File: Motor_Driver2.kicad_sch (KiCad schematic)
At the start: 20 parts, among them J701 Conn_01x02_Socket, U701 DMHT6016LFJ-13, U702 DRV8701

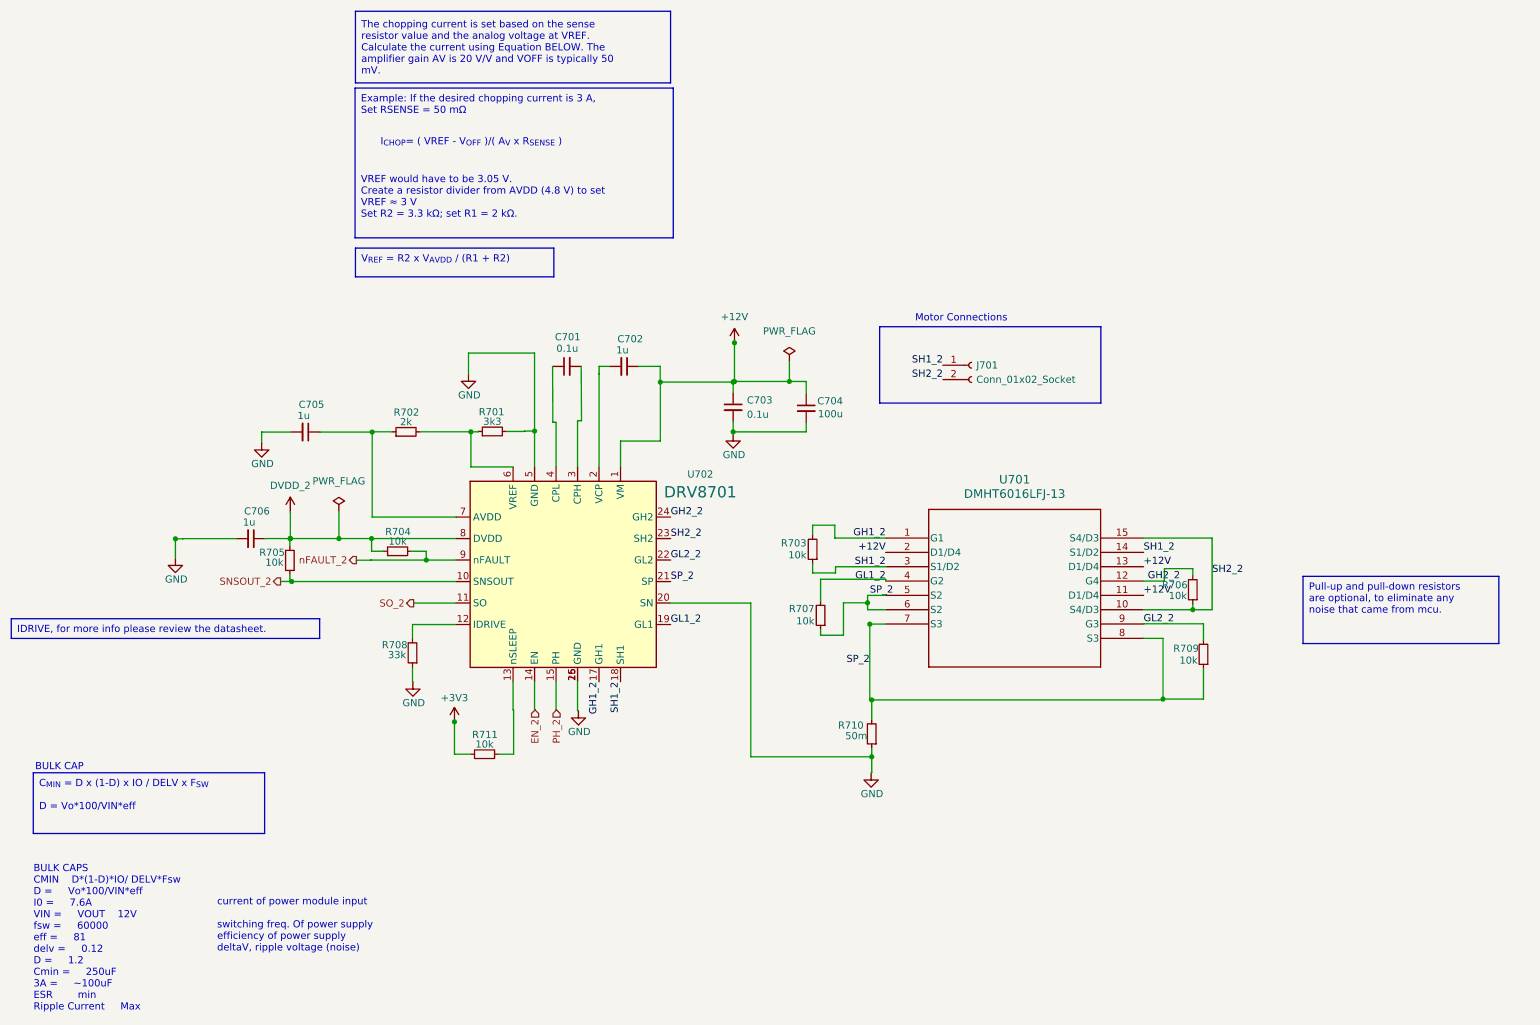
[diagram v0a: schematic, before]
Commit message: schematic pages are reviewed
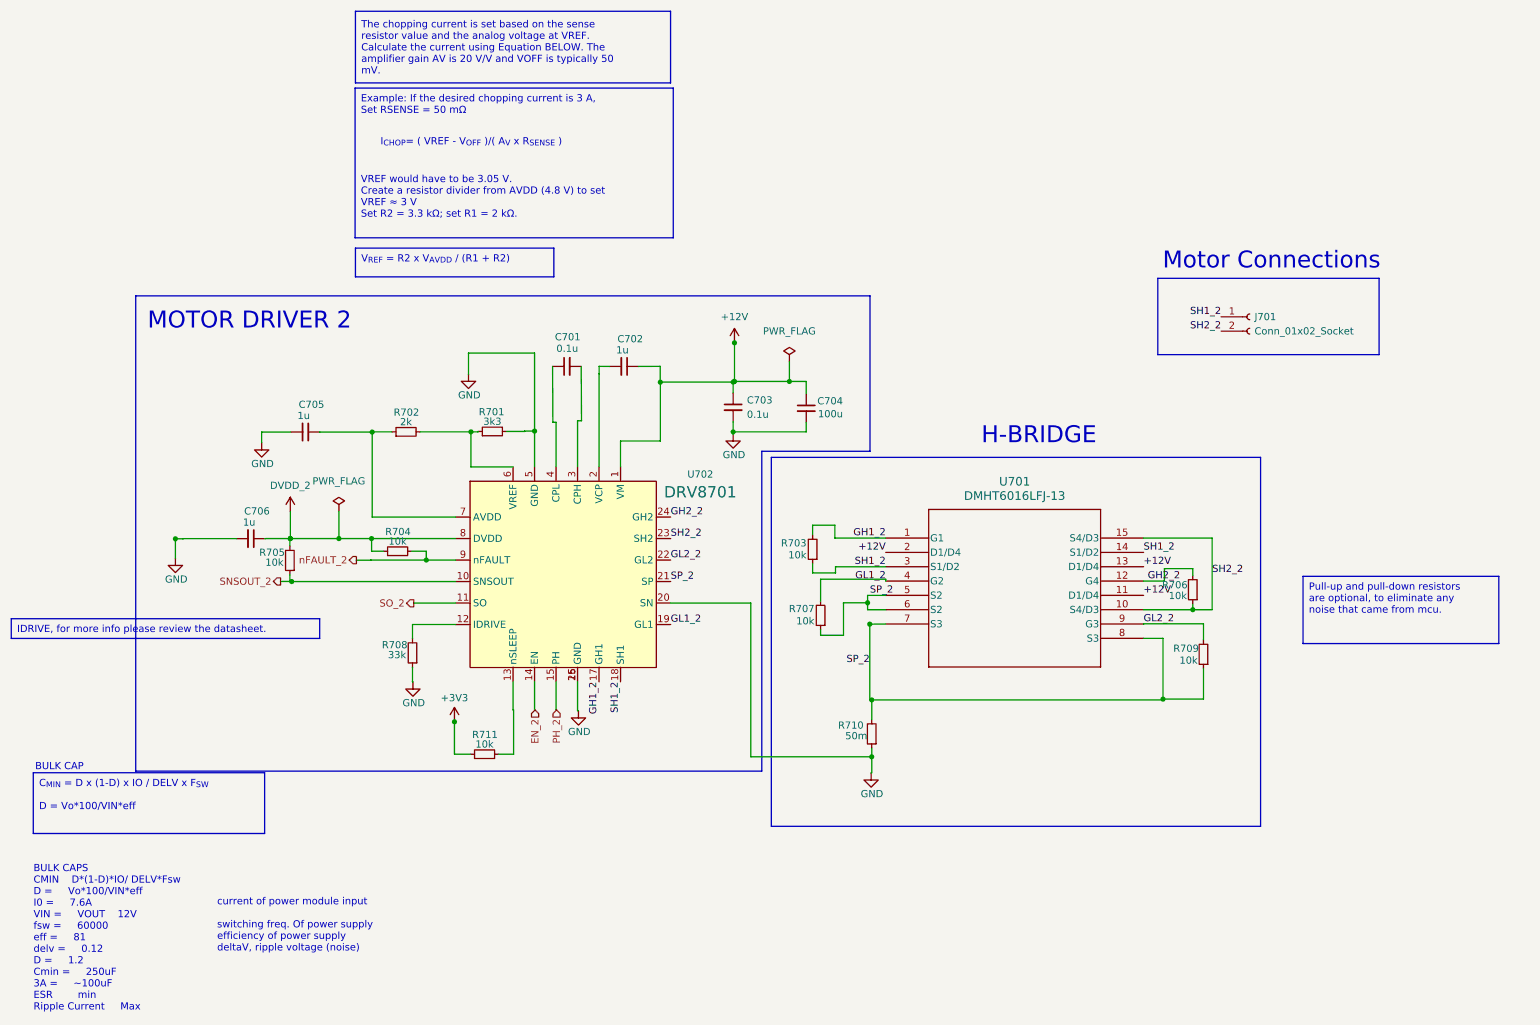
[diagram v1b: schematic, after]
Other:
- note added: "H-BRIDGE"
- note added: "MOTOR DRIVER 2"
- moved on the sheet: J701
